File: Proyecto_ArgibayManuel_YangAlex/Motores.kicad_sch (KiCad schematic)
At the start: 10 parts, among them K1 RT314012, K2 RT314012, Q1 2N2222, Q2 2N2222, U6 DRV8871DDA, U7 DRV8871DDA

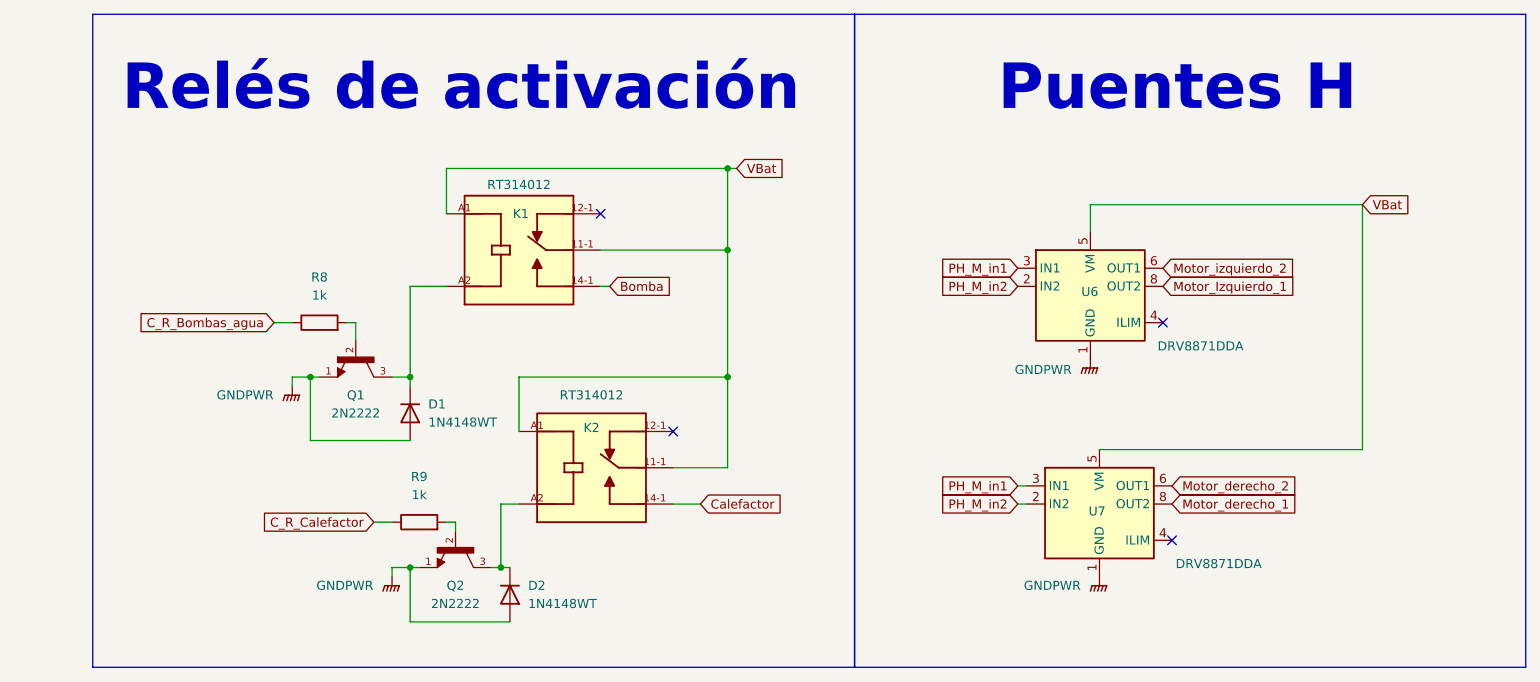
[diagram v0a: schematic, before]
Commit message: Arreglo layout y esqumatico con las correcciones pasadas
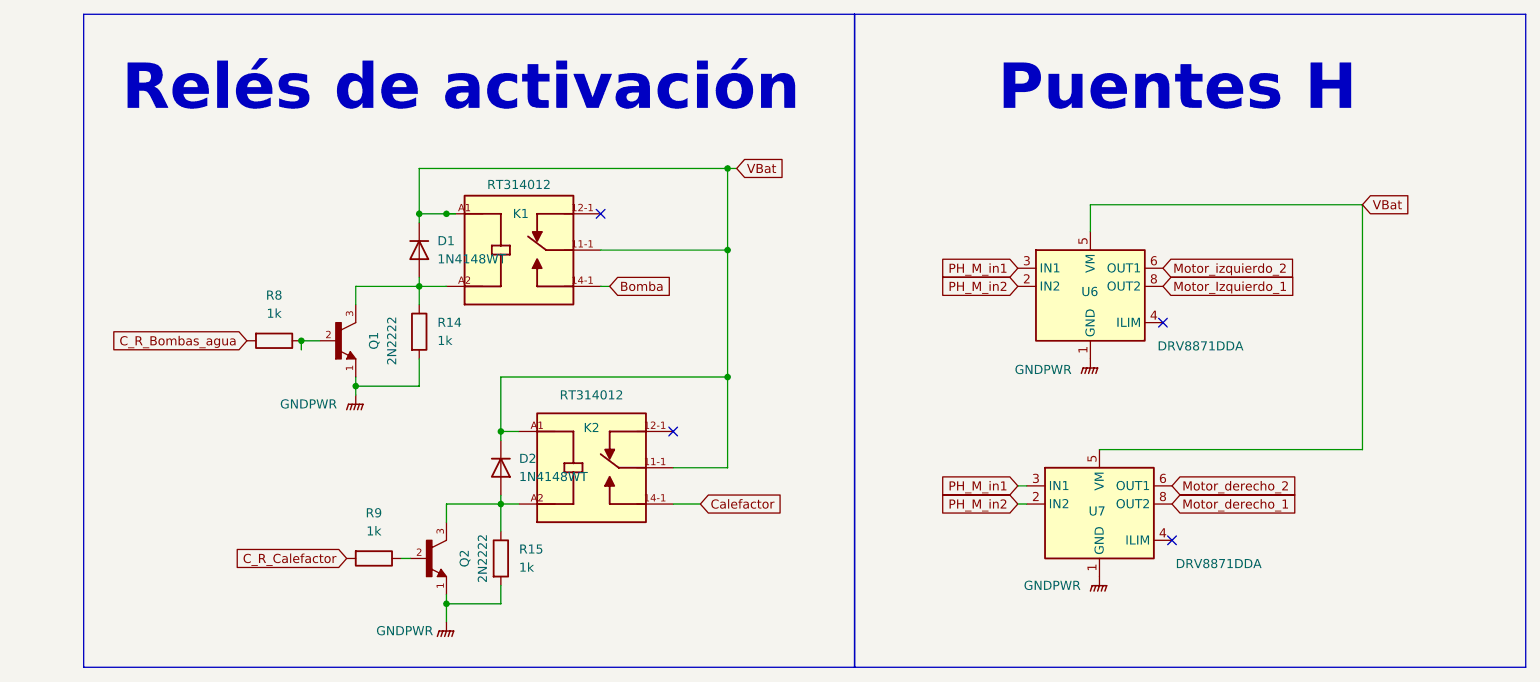
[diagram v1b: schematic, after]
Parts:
- added R14, R15: 1k, Resistor_SMD:R_0805_2012Metric, symbol Device:R
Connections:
- net C_R_Bombas_agua: now also R8.2; no longer R8.1
- net C_R_Calefactor: now also R9.2; no longer R9.1
- net GNDPWR: now also R14.2, R15.2; no longer D1.2 (A), D2.2 (A)
- net VBat: now also D1.1 (K), D2.1 (K)
- net at K2.A2, Q2.3: now also D2.2 (A), R15.1; no longer D2.1 (K)
- net at Q1.2: now also R8.1; no longer R8.2
- net at K1.A2, Q1.3: now also D1.2 (A), R14.1; no longer D1.1 (K)
- net at Q2.2: now also R9.1; no longer R9.2
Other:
- moved on the sheet: D1, D2, Q1, Q2, R8, R9
